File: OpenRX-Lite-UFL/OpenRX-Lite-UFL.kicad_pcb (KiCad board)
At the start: 6 copper layers, 8.2 x 12.2 mm, 39 parts, among them U1 ESP32-C3FH4, U2 TLV75533PDQNR, U3 SX1281IMLTRT, X1 CJ17-400001010B20

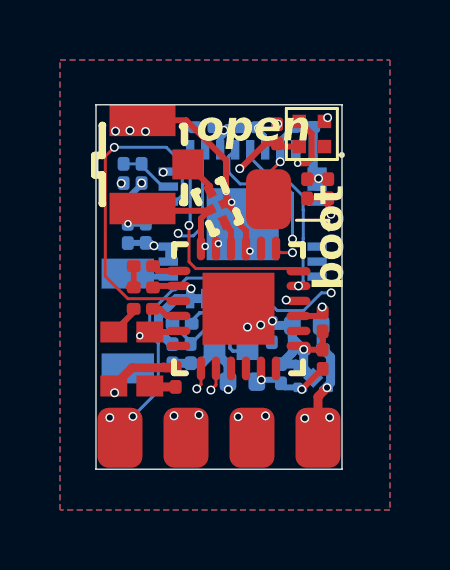
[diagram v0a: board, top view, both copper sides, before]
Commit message: initial routing for all
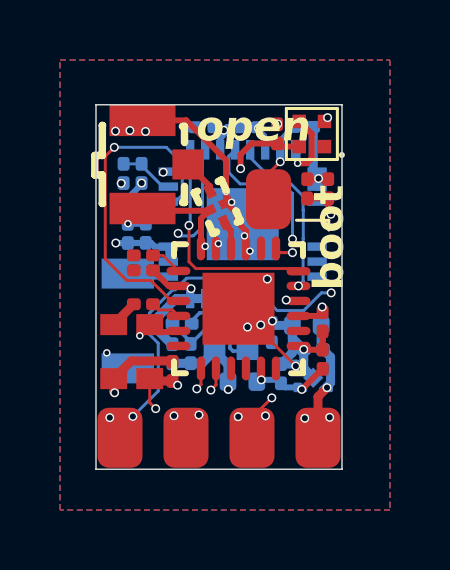
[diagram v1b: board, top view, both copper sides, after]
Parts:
- moved C14 0.57 mm to (180.8, 96.1)
- moved C20 0.36 mm to (180.8, 95.6)
- moved OSC1 0.25 mm to (180.4, 98.8)
- moved C13 0.22 mm to (181.8, 99.4)
- moved C19 0.16 mm to (180.8, 97.2)
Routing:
- net GND: track 39.0 -> 45.8 mm, vias 23 -> 29
- net +3V3: track 19.8 -> 21.5 mm
- net unconnected-(AE1-Pad2): vias 0 -> 1
